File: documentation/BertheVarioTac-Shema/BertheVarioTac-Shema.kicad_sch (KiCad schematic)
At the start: 12 parts, among them CN1 4P-1.25 Temperature and humid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, P1 4P-1.25 Power supply base, P1 Potentiometer 10k ohms, P3 4P-1.25 Extended IO, P4 2P-1.25 SPEAK

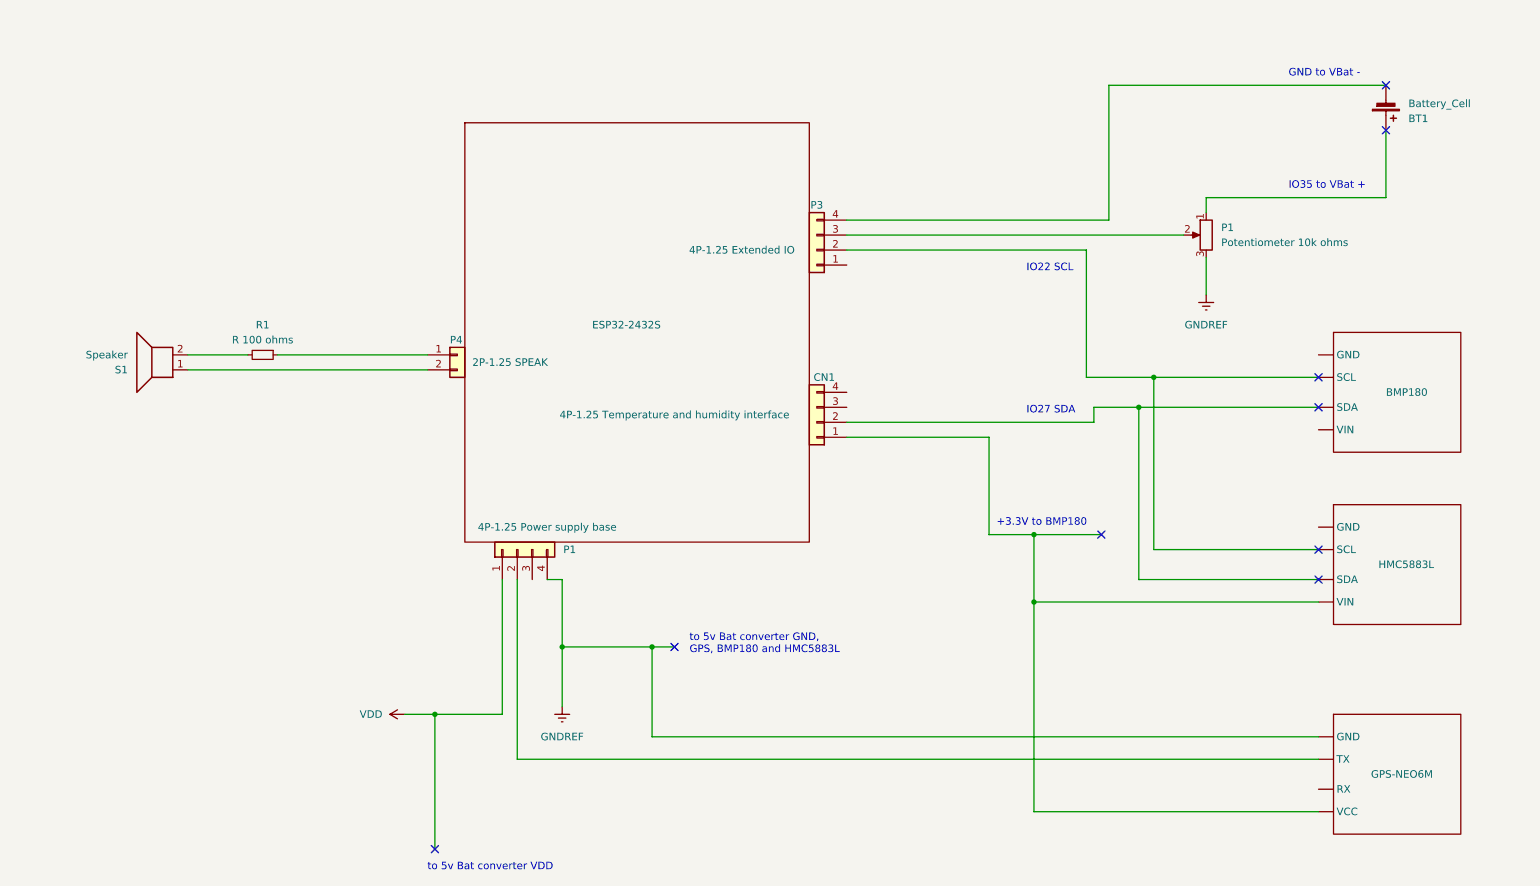
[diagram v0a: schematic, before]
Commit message: mise a jour kicad
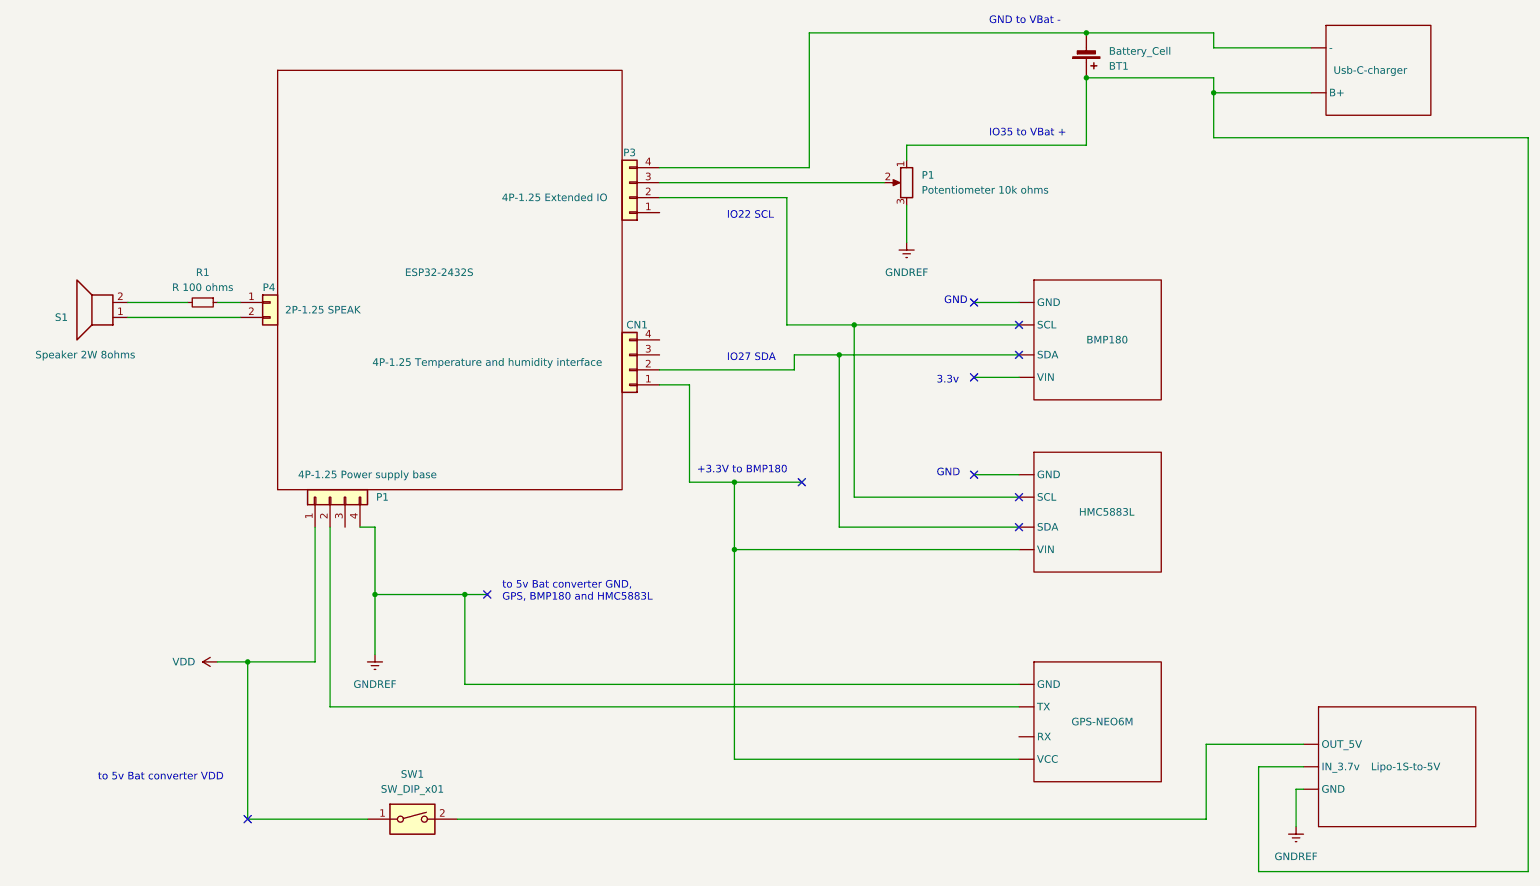
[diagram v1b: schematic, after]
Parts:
- added Lipo-1S-to-5V: ~, symbol BertheLibrary:Lipo-to-5v
- added SW1: SW_DIP_x01, symbol Switch:SW_DIP_x01
- added Usb-C-charger: ~, symbol BertheLibrary:Usb_c_charger
- S1: value Speaker -> Speaker 2W 8ohms
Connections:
- net GNDREF: now also Lipo-1S-to-5V. (OUT_5V)
- net VDD: now also SW1.1
- net at HMC5883L. (VIN): now also CN1.1 (Pin_1), GPS-NEO6M. (VCC)
- net at BT1.1 (+), P1.1: now also Lipo-1S-to-5V. (OUT_5V), Usb-C-charger. (B+)
- net at BT1.2 (-), P3.4 (Pin_4): now also Usb-C-charger. (B+)
- new net: BMP180. (VIN), CN1.2 (Pin_2), HMC5883L. (VIN)
- new net: BMP180. (VIN), HMC5883L. (VIN), P3.2 (Pin_2)
- new net: Lipo-1S-to-5V. (OUT_5V), SW1.2
- now unconnected: BMP180. (VIN), BMP180. (VIN)
- no-connect marks 9 -> 10
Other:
- note added: "3.3v"
- note added: "GND"
- moved on the sheet: BMP180, BT1, CN1, ESP32-2432S, GPS-NEO6M, HMC5883L, P1, P3, P4, R1, S1
